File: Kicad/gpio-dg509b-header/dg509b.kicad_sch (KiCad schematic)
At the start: 8 parts, among them K1 GPIO IN, K2 I/O, K3 I/O, U1 DG509BEY, U2 3M-SJ5376

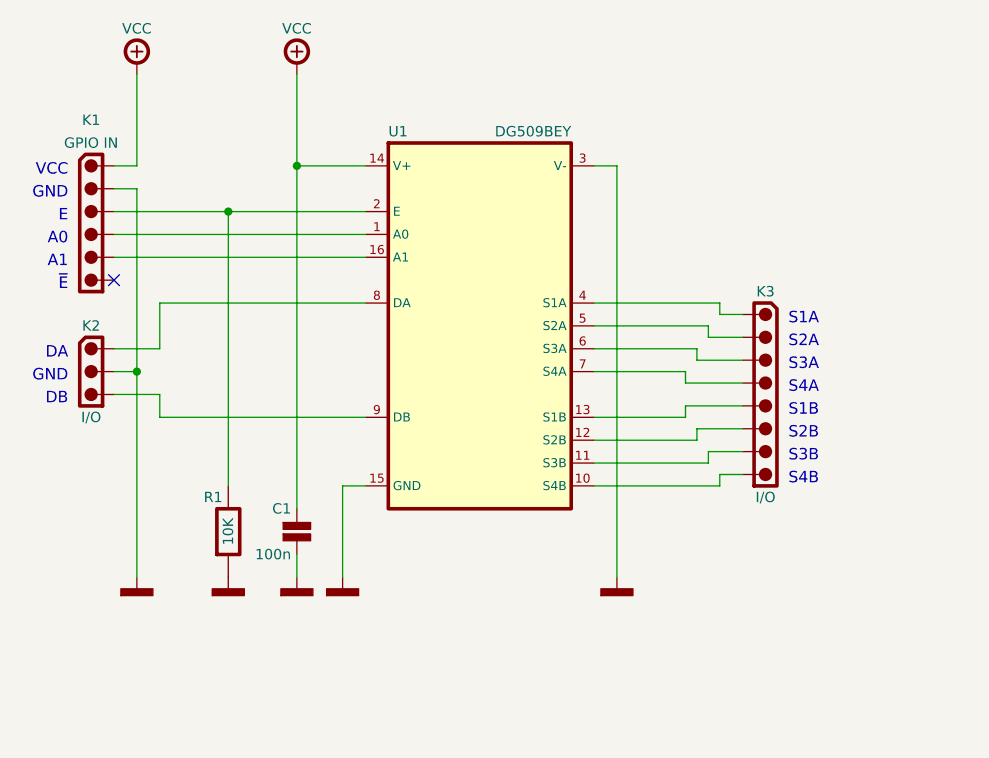
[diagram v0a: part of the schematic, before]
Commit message: Up
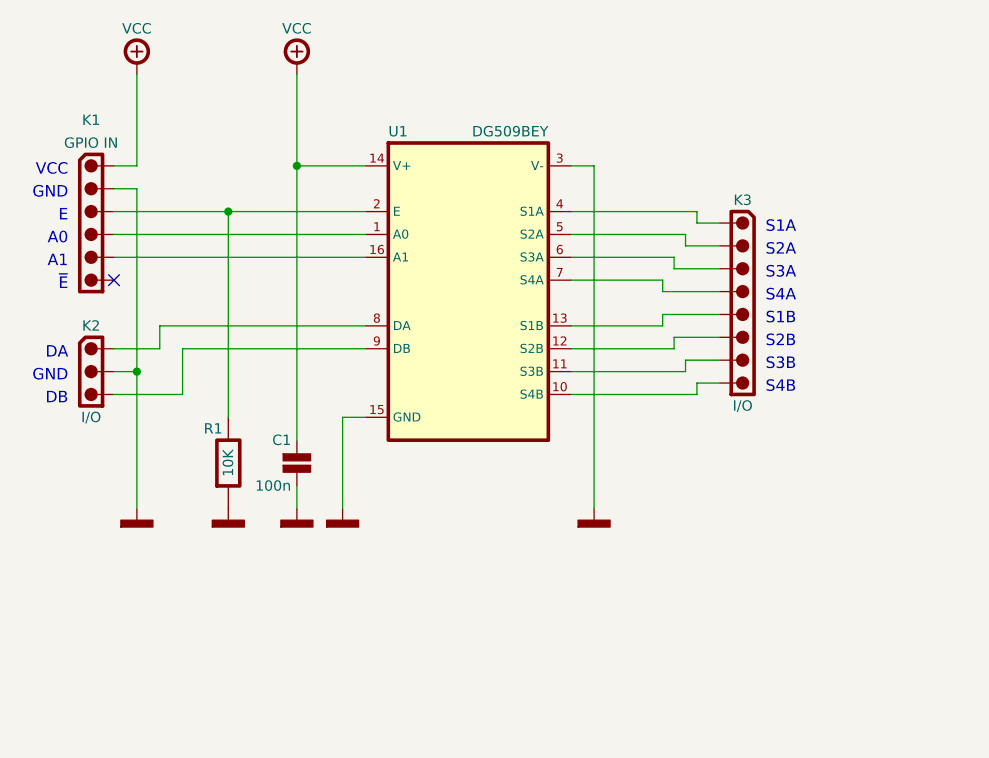
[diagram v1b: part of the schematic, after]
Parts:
- C1: symbol tronixio:CAPACITOR-1206-100N -> tronixio:CAPACITOR-1206-100N-50V-5P-X7R; Mouser 80-C1206C104M5R -> 80-C1206C104J5R; Name CAPACITOR-1206-100N -> (none); Tolerance 20% -> 5%
- K1: Name HARWIN-254-M-1X06-RIGHT-ANGLE -> (none)
- K2: Name HARWIN-254-M-1X03-VERTICAL -> (none)
- K3: Name HARWIN-254-M-1X08-VERTICAL -> (none)
- R1: symbol tronixio:RESISTOR-1206-10K -> tronixio:RESISTOR-1206-10K-5P; Name RESISTOR-1206-10K -> (none)
- TP1: Name KEYSTONE-2000-3 -> (none)
- U1: symbol tronixio:VISHAY-DG509BEY-SOIC-16 -> tronixio:VISHAY-DG509BEY-SOIC; Name VISHAY-DG509BEY-SOIC-16 -> (none)
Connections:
- net VCC renamed +VCC
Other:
- moved on the sheet: C1, K3, R1, U1
